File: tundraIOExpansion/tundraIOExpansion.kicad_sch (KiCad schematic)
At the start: 26 parts, among them J1 Conn_01x25, J2 Conn_ARM_SWD_TagConnect_TC203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, U1 RP2040, U2 MX25L3233FM2, U3 TCA9544A, Y1 Crystal

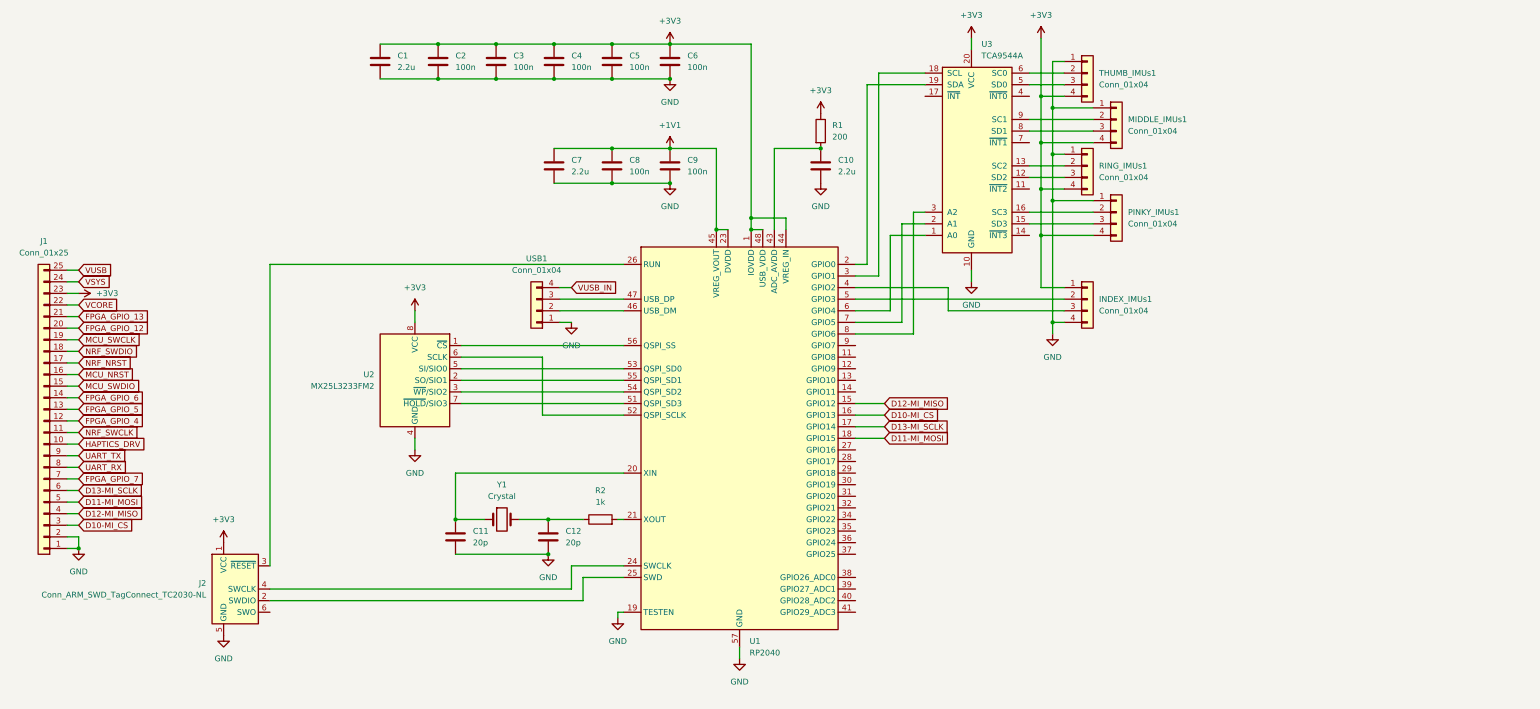
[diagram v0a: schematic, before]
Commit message: Updating main interface board
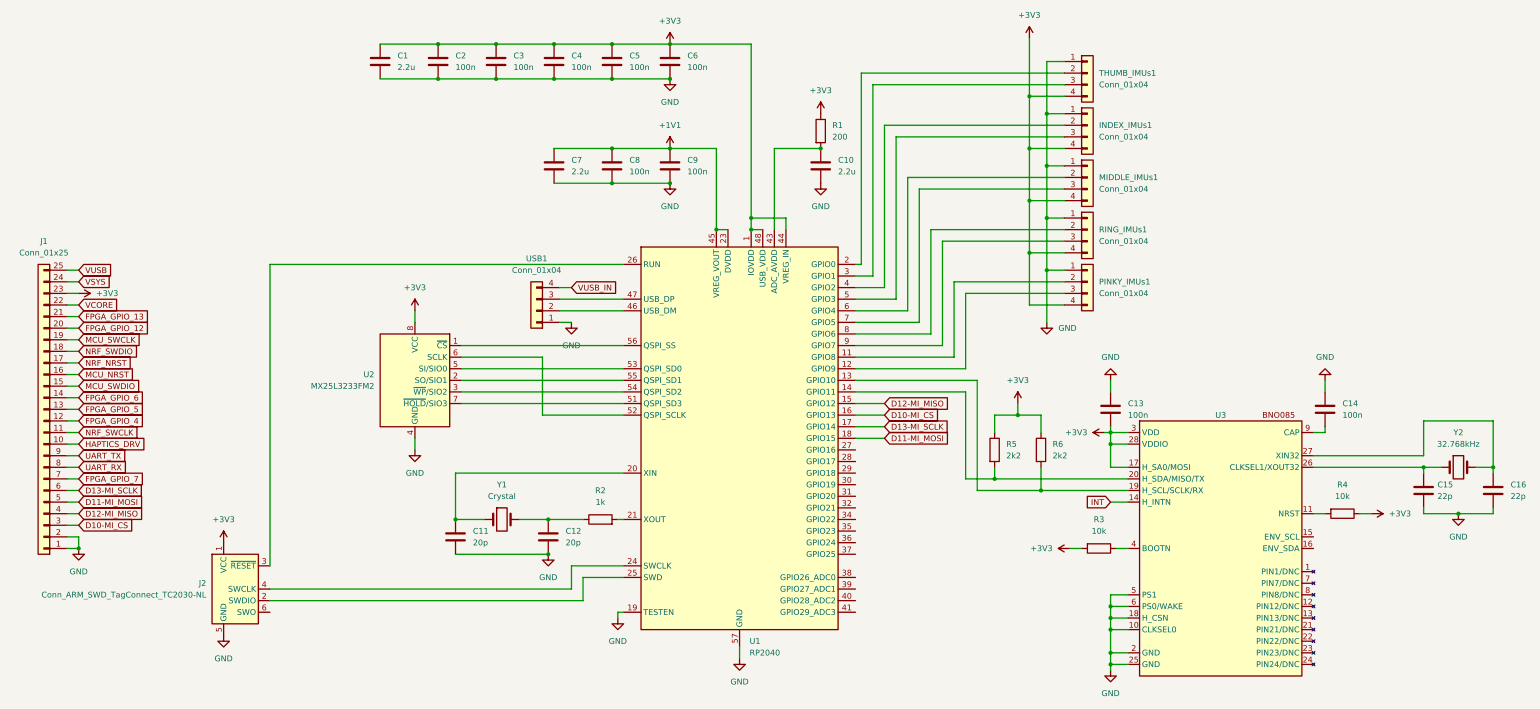
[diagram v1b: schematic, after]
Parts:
- removed U3: TCA9544A, Package_SO:TSSOP-20_4.4x6.5mm_P0.65mm, symbol Interface_Expansion:TCA9544A
- added C13, C14: 100n, Capacitor_SMD:C_0603_1608Metric, symbol Device:C
- added C15, C16: 22p, Capacitor_SMD:C_0603_1608Metric, symbol Device:C
- added R3, R4: 10k, Resistor_SMD:R_0603_1608Metric, symbol Device:R
- added R5, R6: 2k2, Resistor_SMD:R_0603_1608Metric, symbol Device:R
- added U3: ~, Package_LGA:LGA-28_5.2x3.8mm_P0.5mm, symbol IMUs:BNO085
- added Y2: 32.768kHz, Crystal:Crystal_SMD_3215-2Pin_3.2x1.5mm, symbol Device:Crystal
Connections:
- net +3V3: now also INDEX_IMUs1.4 (Pin_4), C13.2, R3.2, R4.1, R5.1, R6.1, U3.17 (H_SA0/MOSI), U3.28 (VDDIO), U3.3 (VDD); no longer INDEX_IMUs1.1 (Pin_1)
- net GND: now also INDEX_IMUs1.1 (Pin_1), C13.1, C14.1, C15.2, C16.2, U3.10 (CLKSEL0), U3.18 (H_CSN), U3.2 (GND), U3.25 (GND), U3.5 (PS1), U3.6 (PS0/WAKE); no longer INDEX_IMUs1.4 (Pin_4)
- net at U1.6 (GPIO4): now also MIDDLE_IMUs1.2 (Pin_2)
- net at RING_IMUs1.3 (Pin_3): now also U1.9 (GPIO7)
- net at RING_IMUs1.2 (Pin_2): now also U1.8 (GPIO6)
- net at PINKY_IMUs1.3 (Pin_3): now also U1.12 (GPIO9)
- net at PINKY_IMUs1.2 (Pin_2): now also U1.11 (GPIO8)
- net at U1.3 (GPIO1): now also THUMB_IMUs1.3 (Pin_3)
- net at U1.2 (GPIO0): now also THUMB_IMUs1.2 (Pin_2)
- net at U1.7 (GPIO5): now also MIDDLE_IMUs1.3 (Pin_3)
- net at U1.13 (GPIO10): now also R6.2, U3.19 (H_SCL/SCLK/RX)
- net at U1.14 (GPIO11): now also R5.2, U3.20 (H_SDA/MISO/TX)
- net at U1.4 (GPIO2): now also INDEX_IMUs1.2 (Pin_2); no longer INDEX_IMUs1.3 (Pin_3)
- net at U1.5 (GPIO3): now also INDEX_IMUs1.3 (Pin_3); no longer INDEX_IMUs1.2 (Pin_2)
- new net: R4.2, U3.11 (NRST)
- new net: C15.1, U3.26 (CLKSEL1/XOUT32), Y2.1
- new net: C16.1, U3.27 (XIN32), Y2.2
- new net: R3.1, U3.4 (BOOTN)
- new net: C14.2, U3.9 (CAP)
- new net INT: U3.14 (H_INTN)
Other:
- moved on the sheet: INDEX_IMUs1, MIDDLE_IMUs1, PINKY_IMUs1, RING_IMUs1
